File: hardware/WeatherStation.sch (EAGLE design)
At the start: 9 parts, among them X2 XRJK-S-01-6-4-0-9M2

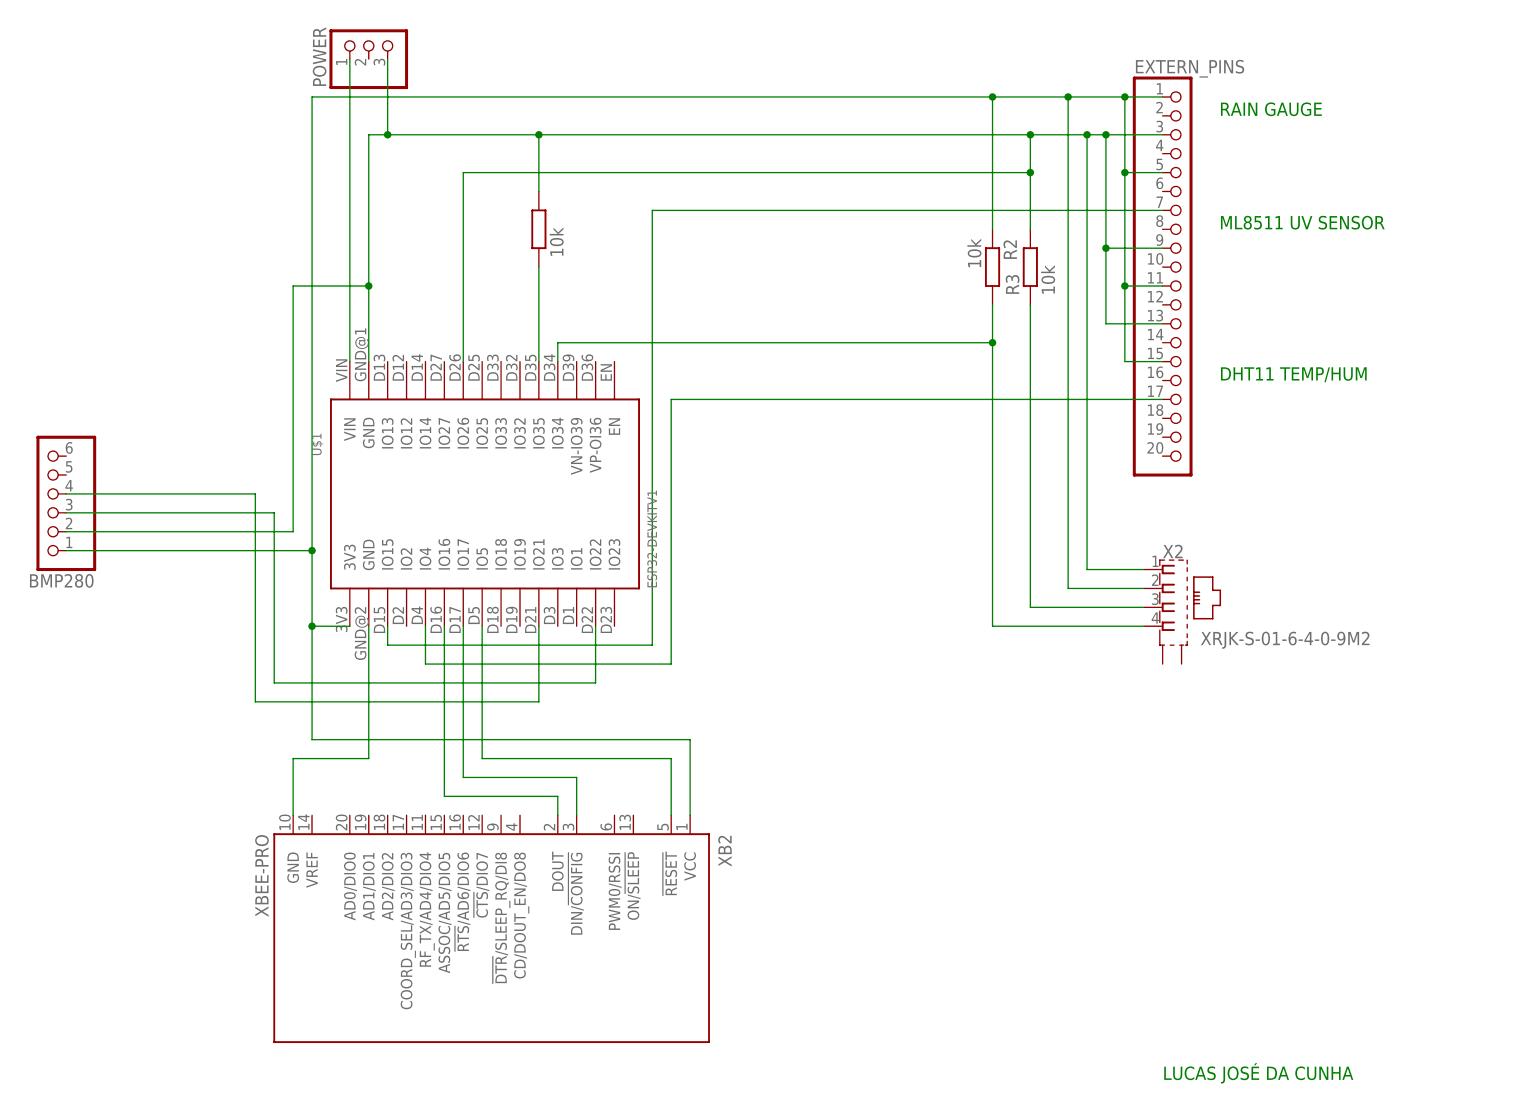
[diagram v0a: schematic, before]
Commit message: fixing schematic v1.1
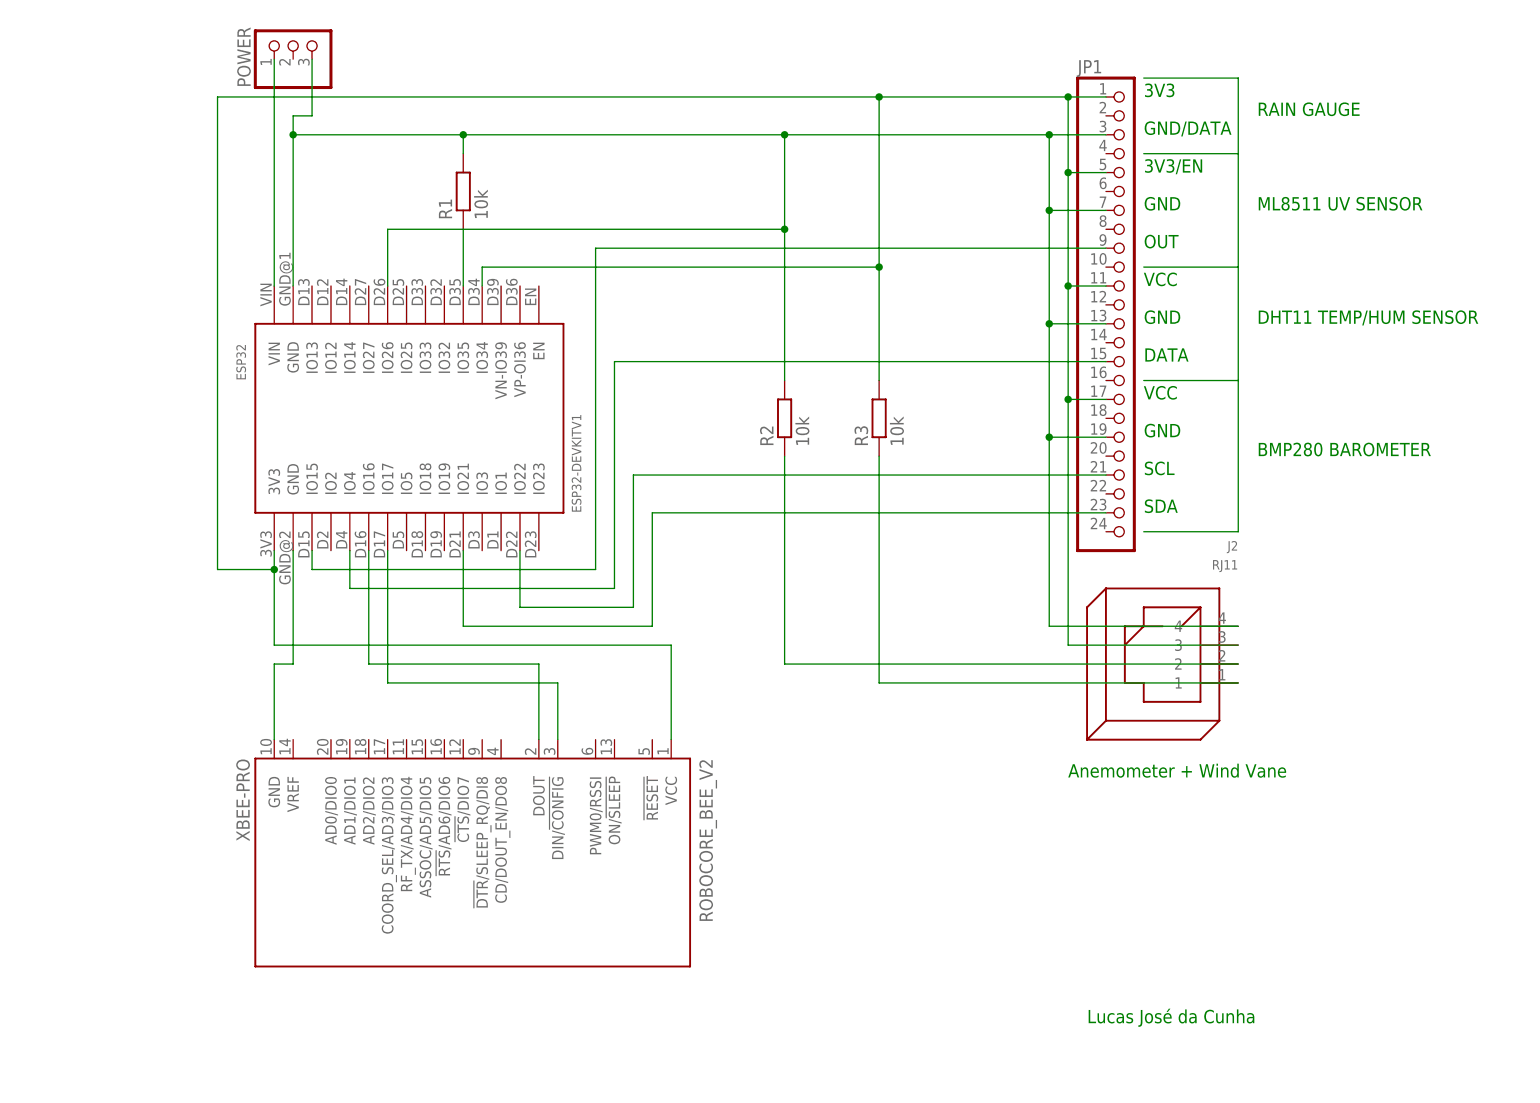
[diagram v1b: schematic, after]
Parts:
- removed BMP280: (no value), pinhead:PINHD-1X6
- removed EXTERN_PINS: (no value), pinhead:PINHD-1X20
- removed U$1: ESP32DEVKITV1, ESP32-DEVKITV1:ESP32DEVKITV1
- removed X2: XRJK-S-01-6-4-0-9M2, con-xmultiplee:XRJK-S-01-6-4-0-9M2
- removed XB2: XBEE-PRO, maxstream:XBEE-PRO
- added ESP32: ESP32DEVKITV1, ESP32-DEVKITV1:ESP32DEVKITV1
- added J2: RJ11, con-rj_fixed:RJ11
- added JP1: (no value), pinhead:PINHD-1X24
- added ROBOCORE_BEE_V2: XBEE-PRO, maxstream:XBEE-PRO
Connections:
- removed net N$13: U$1.IO16, XB2.DOUT
- removed net N$15: U$1.IO5, XB2.!RESET
- new net N$9: ESP32.IO22, JP1.21
- net N$1: now also ESP32.3V3, ESP32.IO34, J2.3, JP1.1, JP1.11, JP1.17, JP1.5, R3.2, ROBOCORE_BEE_V2.VCC; no longer POWER.1, U$1.VIN
- net N$10: now also ESP32.IO21, JP1.23; no longer BMP280.3, U$1.IO22
- net N$11: now also ESP32.IO17, ROBOCORE_BEE_V2.DIN/!CONFIG; no longer BMP280.4, U$1.IO21
- net N$12: now also J2.2, R2.1; no longer U$1.GND@2, XB2.GND
- net N$14: now also J2.1, R3.1; no longer U$1.IO17, XB2.DIN/!CONFIG
- net N$2: now also ESP32.GND@1, ESP32.IO26, J2.4, JP1.13, JP1.19, JP1.3, JP1.7, R2.2; no longer BMP280.2, EXTERN_PINS.13, EXTERN_PINS.3, EXTERN_PINS.9, R3.2, U$1.GND@1, U$1.IO26, X2.1
- net N$3: now also ESP32.IO35, R1.1; no longer BMP280.1, EXTERN_PINS.1, EXTERN_PINS.11, EXTERN_PINS.15, EXTERN_PINS.5, R2.1, U$1.3V3, X2.2, XB2.VCC
- net N$4: now also ESP32.IO15, JP1.9; no longer R1.1, U$1.IO35
- net N$5: now also ESP32.IO16, ROBOCORE_BEE_V2.DOUT; no longer EXTERN_PINS.7, U$1.IO15
- net N$6: now also ESP32.GND@2, ROBOCORE_BEE_V2.GND; no longer EXTERN_PINS.17, U$1.IO4
- net N$7: now also ESP32.IO4, JP1.15; no longer R2.2, U$1.IO34, X2.4
- net N$8: now also ESP32.VIN, POWER.1; no longer R3.1, X2.3
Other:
- note added: "3V3"
- note added: "3V3/EN"
- note added: "Anemometer + Wind Vane"
- note added: "BMP280 BAROMETER"
- note added: "DATA"
- note added: "DHT11 TEMP/HUM SENSOR"
- note added: "GND"
- note added: "GND/DATA"
- note added: "Lucas José da Cunha"
- note added: "OUT"
- note added: "SCL"
- note added: "SDA"
- note added: "VCC"
- note removed: "DHT11 TEMP/HUM"
- note removed: "LUCAS JOSÉ DA CUNHA"
- moved on the sheet: POWER, R2, R3
